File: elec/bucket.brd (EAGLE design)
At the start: 65 x 56 mm, 4 parts, among them U1 PCF85263ATT/AJ-SO8

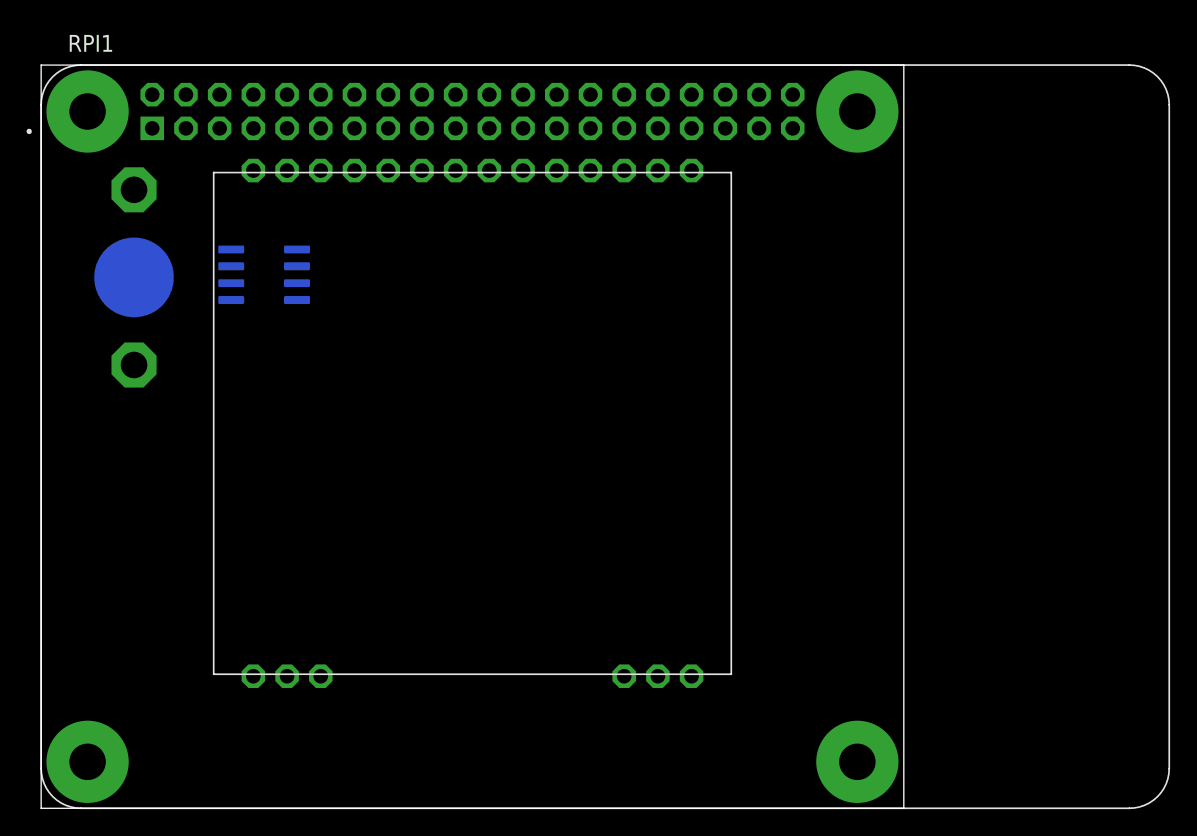
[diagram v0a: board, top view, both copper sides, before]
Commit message: major progress on circuit design
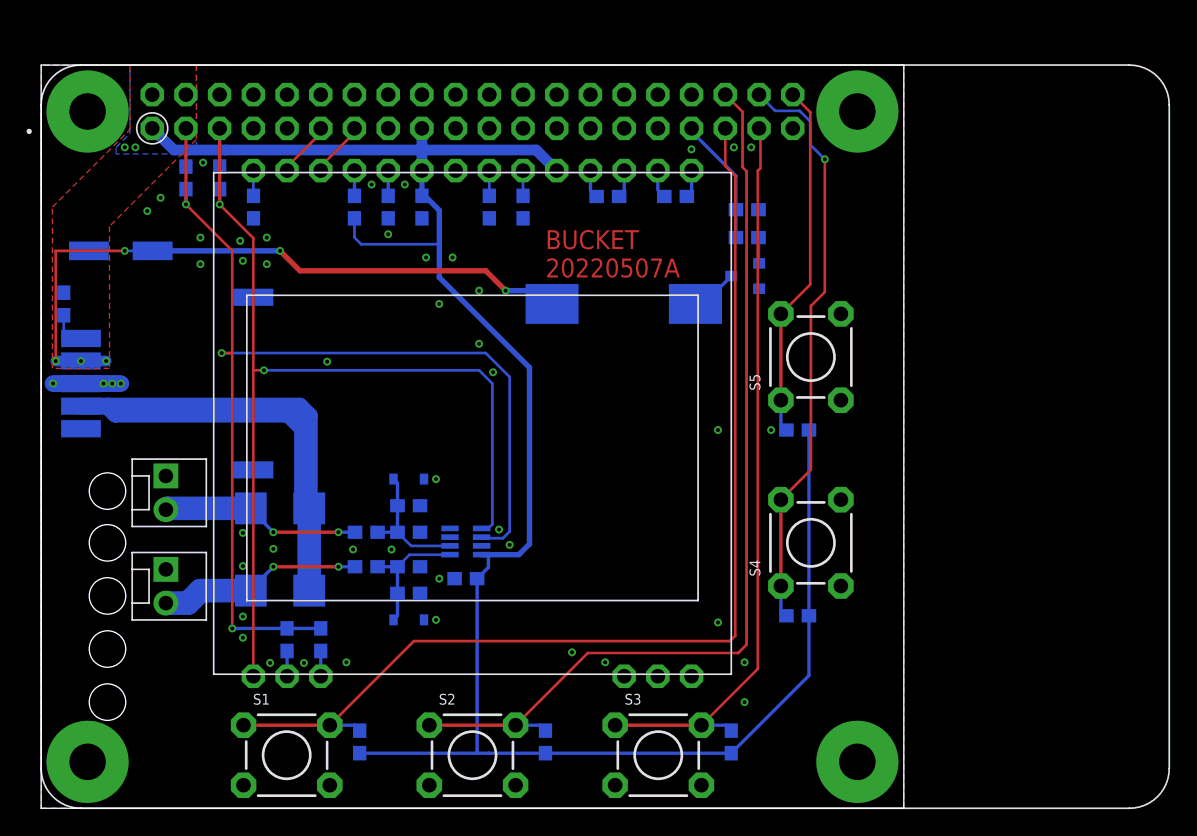
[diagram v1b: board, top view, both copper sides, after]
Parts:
- removed BAT1: BATT-COIN-KEYSTONE-3001, bucket:COIN-KEYSTONE-3001
- removed U1: PCF85263ATT/AJ-SO8, bucket:SOIC127P600X175-8N
- added C1: 47uF, bucket:PANASONIC_D
- added C2, C9: 100nF, bucket:0603-CAP
- added C3, C4: 2u2, bucket:0603-CAP
- added C5, C6, C7, C8: 1uF, bucket:0603-CAP
- added D1, D2: (no value), bucket:SMB-DIODE
- added D3, D4: 2V4, bucket:SOD-323
- added IC1: PSU-OKRT6, bucket:PSU-OKRT6
- added JP1, JP2: (no value), bucket:MOLEX-1X2
- added LS1: CT-1205C-SMT, bucket:CUI_CT-1205C-SMT
- added Q1: MOSFET-NCHAN, bucket:SOT23-3
- added R1, R13, R14, R15, R16, R17, R18, R19, R2, R5, R7: 4K7, bucket:0603-RES
- added R10, R11, R12, R8, R9: 0R, bucket:0603-RES
- added R3: 267R, bucket:0603-RES
- added R4, R6: 15K, bucket:0603-RES
- added S1, S2, S3, S4, S5: (no value), bucket:TACTILE-PTH
- added U2: MAX1037EKA, bucket:21-0078H
- RPI1: value RASPBERRY_PI_3_MODEL_B+ -> RASPBERRY PI
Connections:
- removed net +: BAT1.POS1
- removed net +1: BAT1.POS2
- removed net -: BAT1.NEG
- removed net 3V3: RPI1.1, RPI1.17
- removed net 5V0: RPI1.2, RPI1.4
- removed net SHIELD: RPI1.S1, RPI1.S2, RPI1.S3, RPI1.S4
- removed net VBAT: U1.3
- removed net VDD: U1.8
- removed net VSS: U1.4
- new net 3.3V: C2.1, C9.2, OLED1.19, OLED1.23, R1.2, R11.1, R15.2, R16.2, R17.2, R18.2, R19.2, R2.2, RPI1.1, RPI1.17, U2.8
- new net 5V: C1.+, IC1.4, LS1.1, RPI1.2, RPI1.4
- new net ADC-BAT-1: C7.2, D3.1, R6.2, R7.1, U2.1
- new net ADC-BAT-2: C8.1, D4.1, R4.1, R5.2, U2.2
- new net BTN1: R15.1, RPI1.35, S1.1, S1.2
- new net BTN2: R16.1, RPI1.36, S2.1, S2.2
- new net BTN3: R17.1, RPI1.37, S3.1, S3.2
- new net BTN4: R18.1, RPI1.38, S4.1, S4.2
- new net BTN5: R19.1, RPI1.40, S5.1, S5.2
- new net BUZZER: R13.2, R14.1, RPI1.33
- new net N$1: D2.A, JP2.2, R4.2
- new net N$10: OLED1.2, R10.2
- new net N$11: OLED1.25, R11.2
- new net N$12: OLED1.24, R12.2
- new net N$13: C4.1, OLED1.21
- new net N$14: C3.1, OLED1.20
- new net N$16: C5.2, OLED1.18
- new net N$17: C5.1, OLED1.17
- new net N$18: C6.1, OLED1.16
- new net N$19: C6.2, OLED1.15
- new net N$2: D1.A, JP1.2, R6.1
- new net N$3: D1.C, D2.C, IC1.2
- new net N$4: IC1.5, R3.2
- new net N$5: Q1.1, R13.1
- new net N$6: LS1.2, Q1.3
- new net N$7: OLED1.28, R8.2
- new net N$9: OLED1.3, R9.2
- new net OLED-CS: OLED1.26, RPI1.13
- new net OLED-RST: OLED1.27, RPI1.11
- new net SCL: OLED1.1, R2.1, RPI1.5, U2.5
- new net SDA: R1.1, R10.1, R9.1, RPI1.3, U2.6
- net GND: now also C1.-, C2.2, C3.2, C4.2, C7.1, C8.2, C9.1, D3.2, D4.2, IC1.3, JP1.1, JP2.1, OLED1.22, Q1.2, R12.1, R14.2, R3.1, R5.1, R7.2, R8.1, RPI1.S1, RPI1.S2, RPI1.S3, RPI1.S4, S1.3, S1.4, S2.3, S2.4, S3.3, S3.4, S4.3, S4.4, S5.3, S5.4, U2.7
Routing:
- net 3.3V: track 0.00 -> 151.8 mm
- net SDA: track 0.00 -> 84.2 mm, vias 0 -> 3
- net BTN1: track 0.00 -> 80.8 mm
- net SCL: track 0.00 -> 73.4 mm, vias 0 -> 2
- net BTN2: track 0.00 -> 70.9 mm
- net BTN3: track 0.00 -> 55.8 mm
- net N$3: track 0.00 -> 51.4 mm
- net 5V: track 0.00 -> 51.0 mm, vias 0 -> 8
- net BTN4: track 0.00 -> 43.9 mm, vias 0 -> 1
- net BTN5: track 0.00 -> 26.9 mm
- net N$2: track 0.00 -> 15.4 mm, vias 0 -> 2
- net N$1: track 0.00 -> 15.1 mm, vias 0 -> 2
- net ADC-BAT-2: track 0.00 -> 10.0 mm
- net ADC-BAT-1: track 0.00 -> 9.96 mm
- net BUZZER: track 0.00 -> 9.61 mm
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- added copper zone on layer 1, net 5V
- added copper zone on layer 16, net 5V
- added copper zone on layer 1, net GND
- added copper zone on layer 16, net GND
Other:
- board text added: "BUCKET 20220507A"
